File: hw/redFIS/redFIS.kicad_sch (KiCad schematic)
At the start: 71 parts, among them J1 USB_B, J2 DE9_Plug, J3 Conn_01x04, J4 Conn_01x03, Q1 BC850, Q2 BC850, Q3 BC850, Q4 BC857, U1 ESP-32S, U2 AP63203WU, U3 AP63205WU, U4 TJA1049T, U5 CH340G, U6 PCM5102A, U7 AP63203WU, Y1 12Mhz

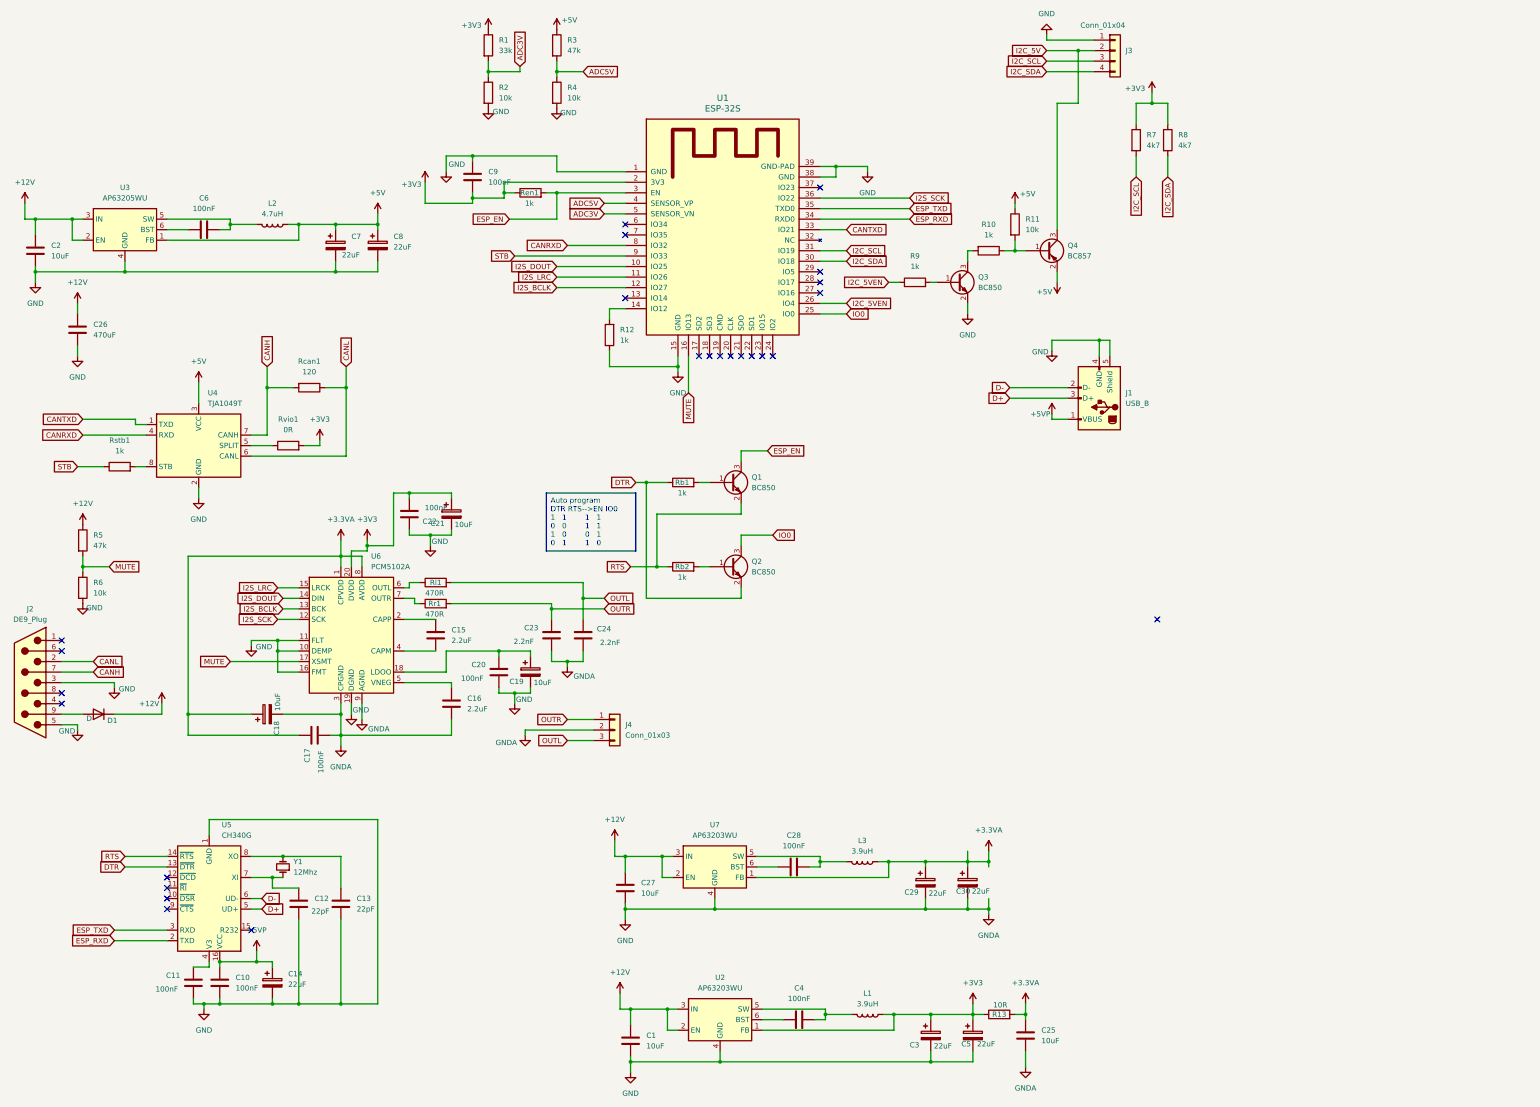
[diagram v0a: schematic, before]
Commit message: HW design bugfix
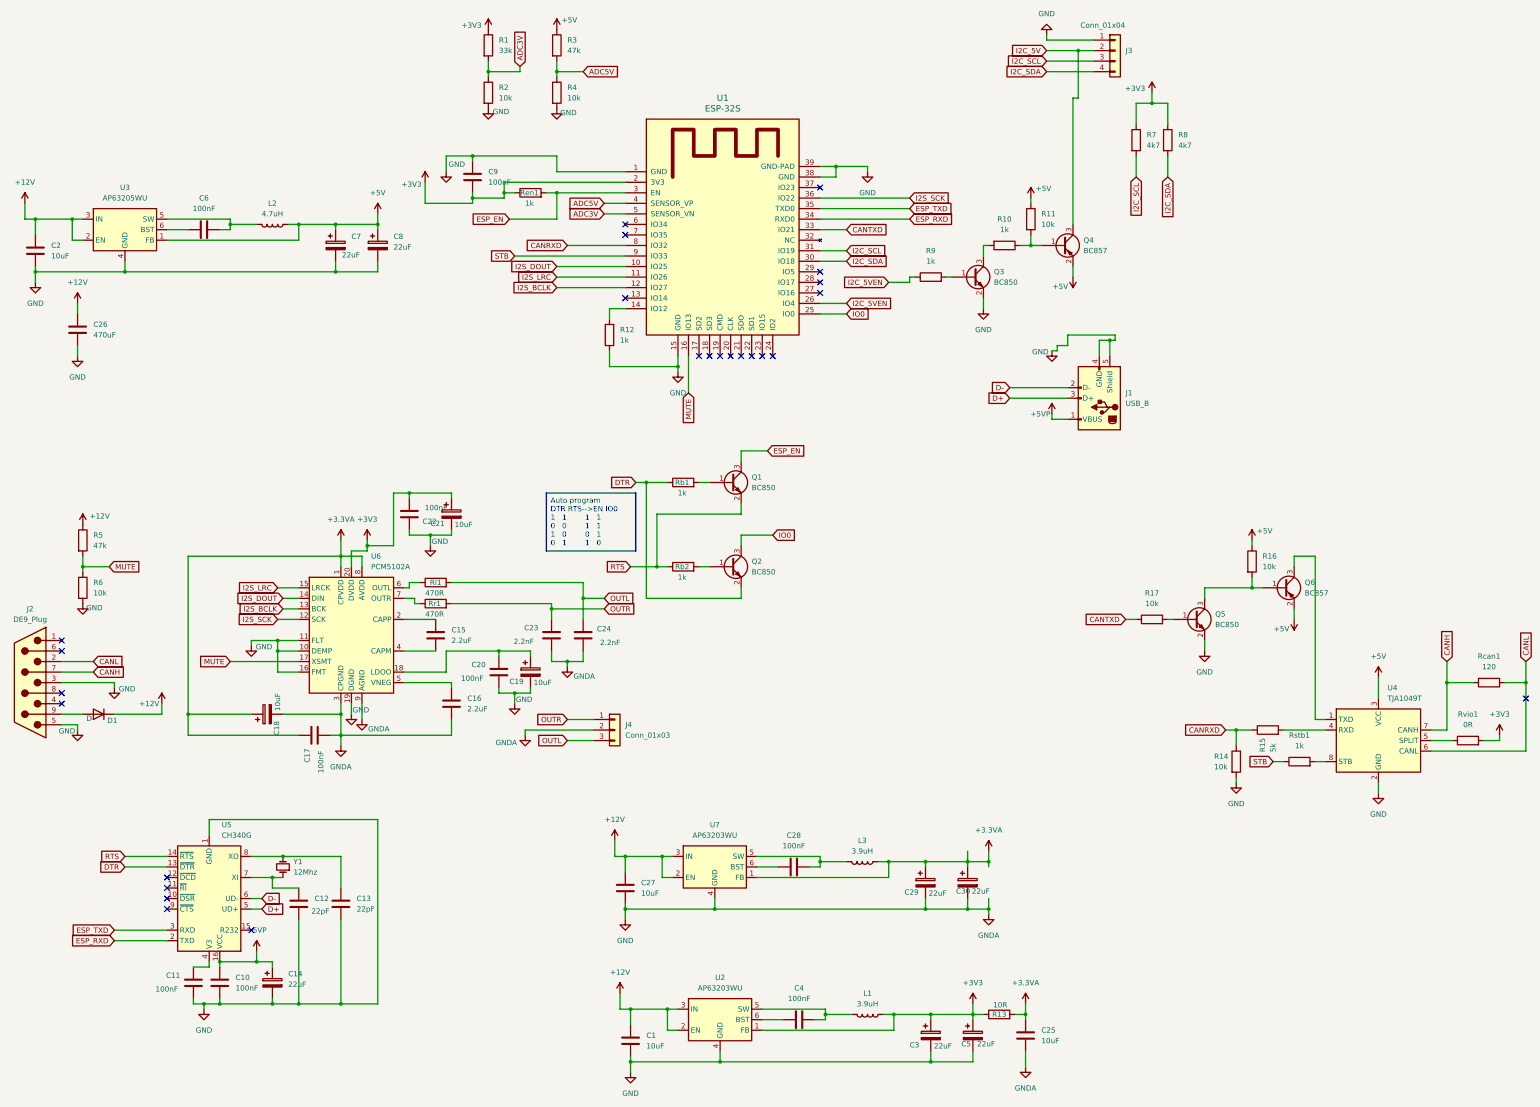
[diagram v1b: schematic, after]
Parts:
- added Q5: BC850, Package_TO_SOT_SMD:SOT-23, symbol Transistor_BJT:BC850
- added Q6: BC857, Package_TO_SOT_SMD:SOT-23, symbol Transistor_BJT:BC857
- added R14, R16, R17: 10k, Resistor_SMD:R_0603_1608Metric_Pad0.98x0.95mm_HandSolder, symbol Device:R
- added R15: 5k, Resistor_SMD:R_0603_1608Metric_Pad0.98x0.95mm_HandSolder, symbol Device:R
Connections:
- net +5V: now also Q6.2 (E), R16.1
- net CANRXD: now also R14.1, R15.1; no longer U4.4 (RXD)
- net CANTXD: now also R17.1; no longer U4.1 (TXD)
- net GND: now also Q5.2 (E), R14.2
- new net: Q5.1 (B), R17.2
- new net: Q5.3 (C), Q6.1 (B), R16.2
- new net: Q6.3 (C), U4.1 (TXD)
- new net: R15.2, U4.4 (RXD)
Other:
- moved on the sheet: Q3, Q4, R10, R11, R9, Rcan1, Rstb1, Rvio1, U4
